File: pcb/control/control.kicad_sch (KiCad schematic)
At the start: 2 parts, among them U1 PicoW, U2 SN65HVD230DR

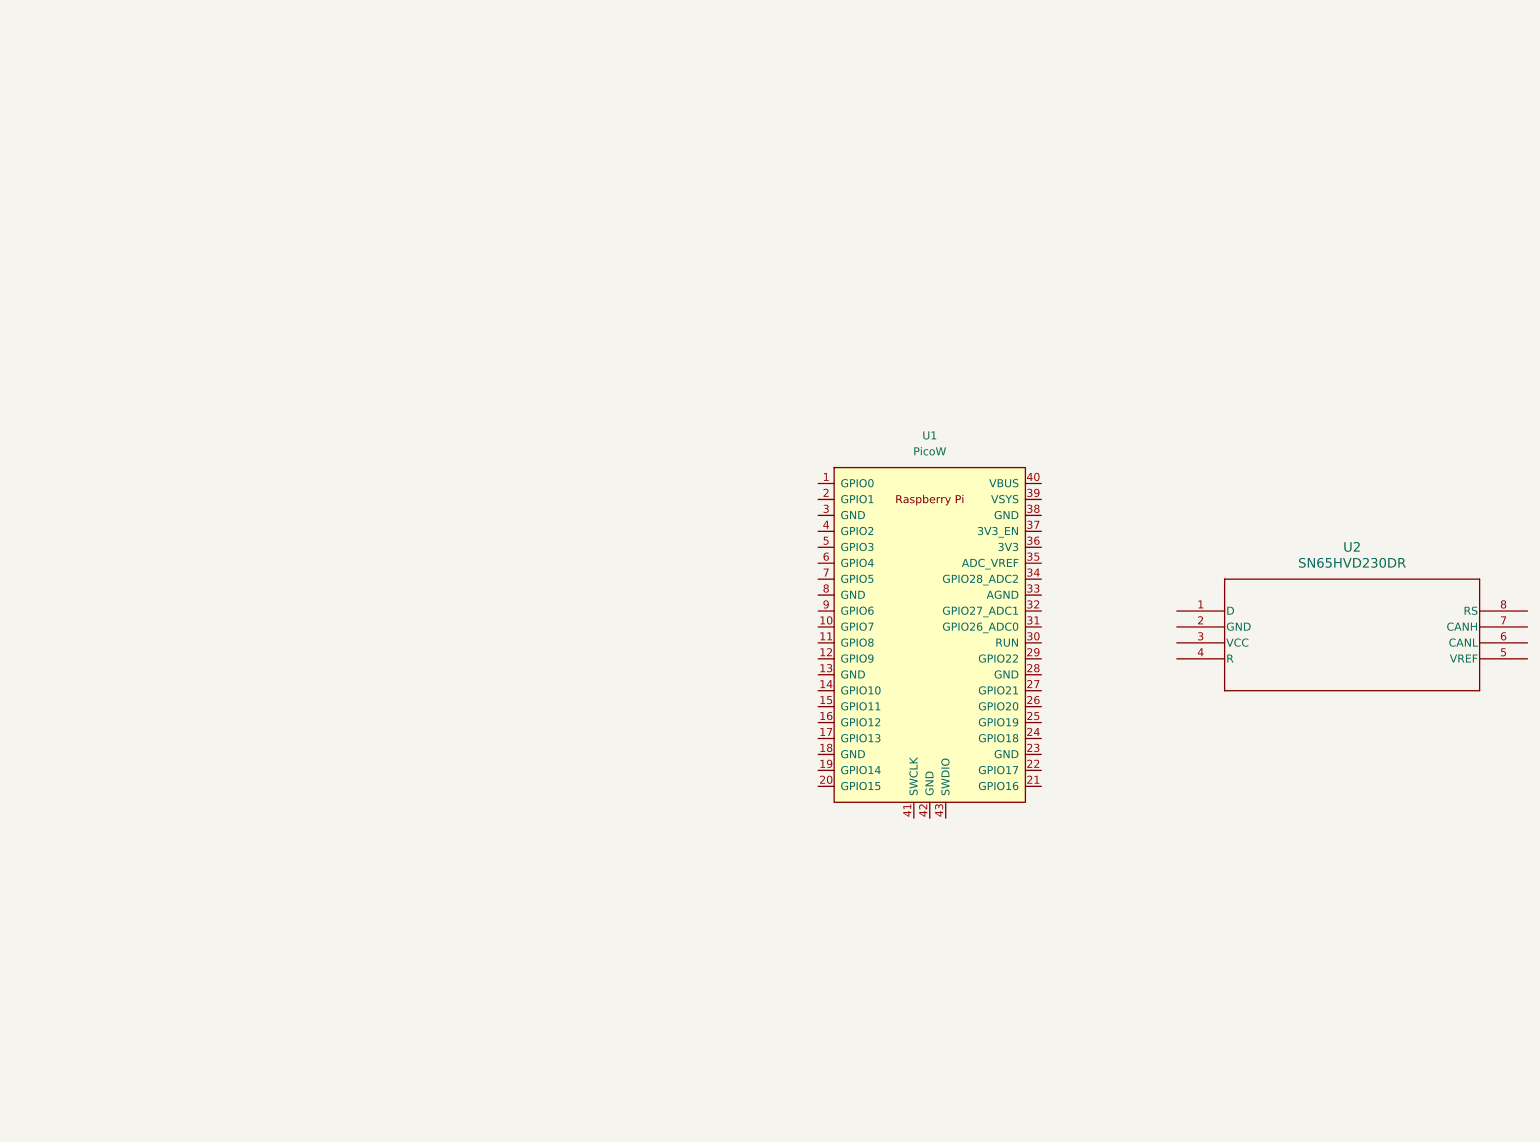
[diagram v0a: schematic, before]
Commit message: Working on control PCB more
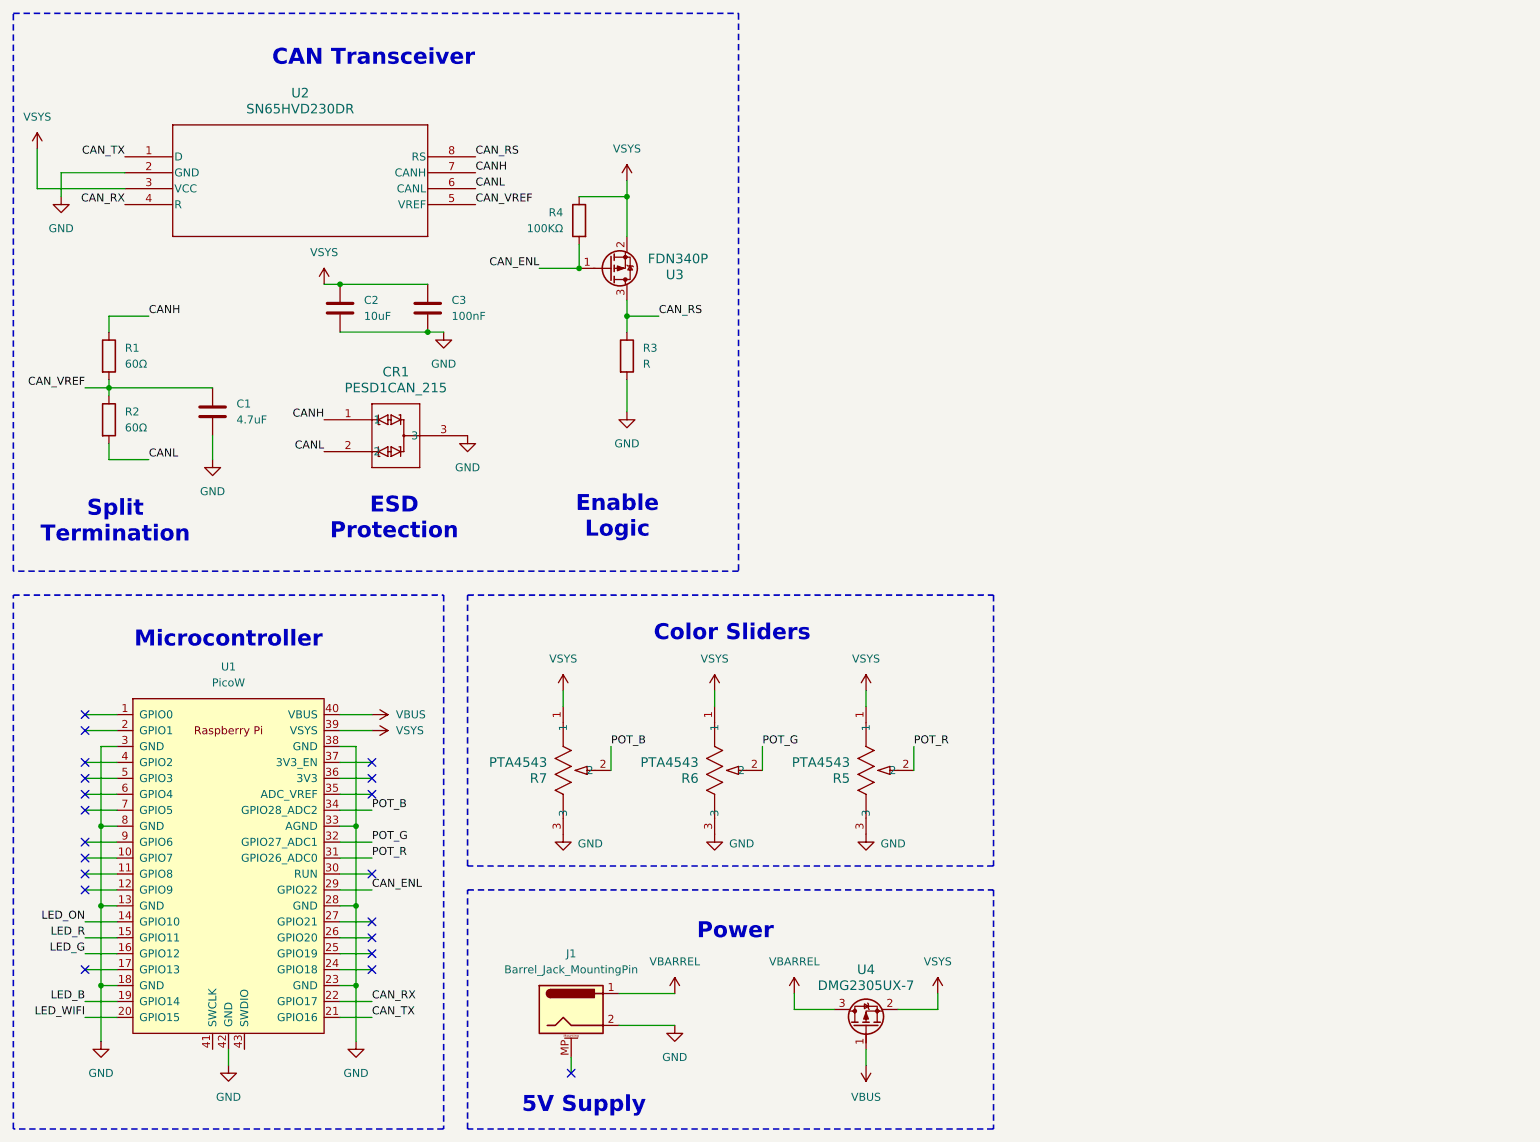
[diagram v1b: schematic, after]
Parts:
- added C1: 4.7uF, symbol Device:C
- added C2: 10uF, symbol Device:C
- added C3: 100nF, symbol Device:C
- added CR1: PESD1CAN_215, pesd:SOT23_PESD1_NEX, symbol pesd:PESD1CAN_215
- added J1: Barrel_Jack_MountingPin, Connector_BarrelJack:BarrelJack_CUI_PJ-102AH_Horizontal, symbol Connector:Barrel_Jack_MountingPin
- added R1, R2: 60Ω, symbol Device:R
- added R3: R, symbol Device:R
- added R4: 100KΩ, symbol Device:R
- added R5, R6, R7: PTA4543, POT_PTA4543, symbol pta4543:PTA4543-2015DPA103
- added U3: FDN340P, fdn340p:SOT-23_ONS, symbol fdn340p:FDN340P
- added U4: DMG2305UX-7, SOT-23_DIO, symbol dmg2305ux:DMG2305UX-7
- U1: footprint RPi_PicoW:RPi_Pico_SMD_TH -> pico:RPi_PicoW_SMD_TH
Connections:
- net GND: now reaches U1.13 (GND)
- net GND: now also U1.18 (GND), U1.23 (GND), U1.28 (GND), U1.3 (GND), U1.33 (AGND), U1.38 (GND), U1.42 (GND), U1.8 (GND), U2.2 (GND), C1.2, C2.2, C3.2, CR1.3, J1.2, R3.2, R5.3, R6.3, R7.3
- net LED_ON: now reaches U1.14 (GPIO10)
- net LED_R: now reaches U1.15 (GPIO11)
- net LED_G: now reaches U1.16 (GPIO12)
- net LED_B: now reaches U1.19 (GPIO14)
- net LED_WIFI: now reaches U1.20 (GPIO15)
- net CAN_TX: now reaches U1.21 (GPIO16)
- net CAN_TX: now also U2.1 (D)
- net CAN_RX: now reaches U1.22 (GPIO17)
- net CAN_RX: now also U2.4 (R)
- net CAN_ENL: now reaches U1.29 (GPIO22)
- net CAN_ENL: now also R4.2, U3.1
- net POT_R: now reaches U1.31 (GPIO26_ADC0)
- net POT_R: now also R5.2
- net POT_G: now reaches U1.32 (GPIO27_ADC1)
- net POT_G: now also R6.2
- net POT_B: now reaches U1.34 (GPIO28_ADC2)
- net POT_B: now also R7.2
- net VSYS: now reaches U1.39 (VSYS)
- net VSYS: now also U2.3 (VCC), C2.1, C3.1, R4.1, R5.1, R6.1, R7.1, U3.2, U4.2
- net VBUS: now reaches U1.40 (VBUS)
- net VBUS: now also U4.1
- net CAN_VREF: now reaches U2.5 (VREF)
- net CAN_VREF: now also C1.1, R1.2, R2.1
- net CANL: now reaches U2.6 (CANL)
- net CANL: now also CR1.2, R2.2
- net CANH: now reaches U2.7 (CANH)
- net CANH: now also CR1.1, R1.1
- net CAN_RS: now reaches U2.8 (RS)
- net CAN_RS: now also R3.1, U3.3
- new net VBARREL: J1.1, U4.3
- no-connect marks 0 -> 20
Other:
- note added: "5V Supply"
- note added: "CAN Transceiver"
- note added: "Color Sliders"
- note added: "ESD Protection"
- note added: "Enable Logic"
- note added: "Microcontroller"
- note added: "Power"
- note added: "Split Termination"
- moved on the sheet: U1, U2
